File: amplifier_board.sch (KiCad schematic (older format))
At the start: 57 parts, among them J1 VCC (7-14V), J2 AUDIO, J3 GND, J4 speaker, J8 speaker, Q1 SQJ860EP, Q2 Q_NMOS_GSD, Q3 SQJ860EP, U1 AD8038, U2 AD8613, U3 LTC4444-5, U4 AD8468, U5 L7805, U6 LM2776, U7 AD8038, U8 AD8468

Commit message: pcb
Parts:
- removed C1: large, Capacitors_ThroughHole:CP_Radial_D10.0mm_P2.50mm_P5.00mm, symbol amplifier_board-rescue:CP-Device
- removed C3: 100uF, Capacitors_SMD:C_1206_HandSoldering, symbol amplifier_board-rescue:C-Device
- removed J4: speaker, Pin_Headers:Pin_Header_Straight_1x02_Pitch2.54mm, symbol Connector_Generic:Conn_02x01
- removed J8: speaker, Terminal_Blocks:TerminalBlock_bornier-2_P5.08mm, symbol amplifier_board-rescue:Screw_Terminal_01x02-Connector
- removed R1, R2: 220, Resistors_SMD:R_1206_HandSoldering, symbol amplifier_board-rescue:R-Device
- added D4, D5, D6: Schottky, Diodes_SMD:D_SMA-SMB_Universal_Handsoldering, symbol amplifier_board-rescue:D_Schottky-Device
- added J4: A, Wire_Pads:SolderWirePad_single_SMD_5x10mm, symbol Connector:Conn_01x01_Female
- added J5: B, Wire_Pads:SolderWirePad_single_SMD_5x10mm, symbol Connector:Conn_01x01_Female
- added JP1, JP3: Jumper-Device, Pin_Headers:Pin_Header_Straight_1x02_Pitch2.54mm, symbol amplifier_board-rescue:Jumper-Device
- added L2: 10uH, Choke_Toroid_ThroughHole:Choke_Toroid_8x16mm_Vertical, symbol amplifier_board-rescue:L-Device
- added Q4, Q5: SQJ402EP, SMD_Packages:SO-8_PowerPAK_Vishay_Single, symbol amplifier_board-rescue:Si7336ADP-Transistor_FET
- added U9: LTC4444-5, Housings_SSOP:MSOP-8-1EP_3x3mm_Pitch0.65mm, symbol LTC4444-5:LTC4444-5
- C7: value 100uF -> 1.5uF
- C8: value 100uF -> 2.2uF
- J1, J3: footprint Mounting_Holes:MountingHole_4mm_Pad -> Wire_Pads:SolderWirePad_single_SMD_5x10mm
- J2: footprint Pin_Headers:Pin_Header_Straight_1x03_Pitch2.54mm -> Pin_Headers:Pin_Header_Angled_1x02_Pitch2.54mm; symbol amplifier_board-rescue:Conn_01x03-Connector_Generic -> Connector_Generic:Conn_01x02
- Q1, Q3: value SQJ860EP -> SQJ402EP
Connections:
- net GND: now also C7.2, C8.1, D6.2 (A), Q5.1 (S), Q5.2 (S), Q5.3 (S), U9.9 (GND)
- net VCC: now also D4.2 (A), D5.1 (K), Q4.5 (D), U9.3 (VCC)
- net audio_in: now also J2.2 (Pin_2)
- net at Q2.1 (G), U4.1: now also JP1.1; no longer U3.1 (Tinp)
- net at Q2.3 (D), R12.1: now also JP3.1; no longer U3.2 (Binp)
- net at RV3.2, U7.3 (+), U8.4 (-): now also C8.2
- new net: C9.1, J5.1 (Pin_1), L1.2
- new net: JP1.2, U3.1 (Tinp), U9.2 (Binp)
- new net: JP3.2, U3.2 (Binp), U9.1 (Tinp)
- new net: Q5.4 (G), U9.4 (BG)
- new net: C5.1, D5.2 (A), D6.1 (K), L2.1, Q4.1 (S), Q4.2 (S), Q4.3 (S), Q5.5 (D), U9.8 (TS)
- new net: Q4.4 (G), U9.7 (TG)
- new net: C7.1, J4.1 (Pin_1), L2.2
- new net: C5.2, D4.1 (K), U9.6 (VB)
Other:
- moved on the sheet: C16, C25, C6, C9, D1, D2, D3, L1, Q1, Q3, U3

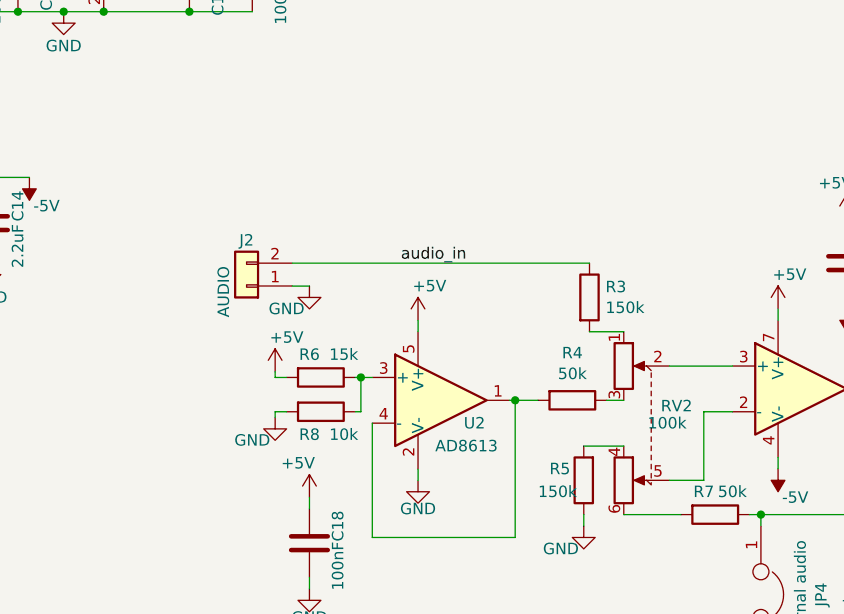
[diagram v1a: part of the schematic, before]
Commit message: pcb improvements
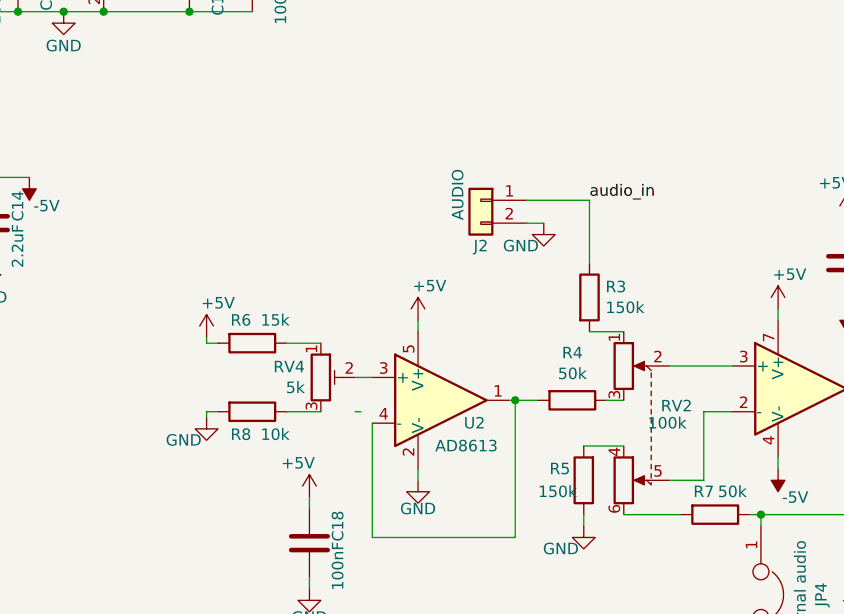
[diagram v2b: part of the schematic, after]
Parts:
- added RV4: 5k, Pin_Headers:Pin_Header_Straight_1x03_Pitch2.54mm, symbol Device:R_POT_TRIM
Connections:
- net GND: now also J2.2 (Pin_2); no longer J2.1 (Pin_1)
- net audio_in: now also J2.1 (Pin_1); no longer J2.2 (Pin_2)
- new net: R6.1, RV4.1
- new net: R8.1, RV4.3
- new net: RV4.2, U2.3 (+)
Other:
- moved on the sheet: J2, R6, R8
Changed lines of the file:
@@
 L amplifier_board-rescue:R-Device R6
 U 1 1 5CA2C628
-P 3375 2825
-F 0 "R6" V 3275 2775 50  0000 C CNN
-F 1 "15k" V 3275 2925 50  0000 C CNN
-F 2 "Resistors_SMD:R_1206_HandSoldering" V 3305 2825 50  0001 C CNN
-F 3 "~" H 3375 2825 50  0001 C CNN
-	1    3375 2825
+P 3075 2675
+F 0 "R6" V 2975 2625 50  0000 C CNN
+F 1 "15k" V 2975 2775 50  0000 C CNN
+F 2 "Resistors_SMD:R_1206_HandSoldering" V 3005 2675 50  0001 C CNN
+F 3 "~" H 3075 2675 50  0001 C CNN
+	1    3075 2675
 	0    1    1    0
 $EndComp
@@
 L amplifier_board-rescue:R-Device R8
 U 1 1 5CA2C63F
-P 3375 2975
-F 0 "R8" V 3475 2925 50  0000 C CNN
-F 1 "10k" V 3475 3075 50  0000 C CNN
-F 2 "Resistors_SMD:R_1206_HandSoldering" V 3305 2975 50  0001 C CNN
-F 3 "~" H 3375 2975 50  0001 C CNN
-	1    3375 2975
+P 3075 2975
+F 0 "R8" V 3175 2925 50  0000 C CNN
+F 1 "10k" V 3175 3075 50  0000 C CNN
+F 2 "Resistors_SMD:R_1206_HandSoldering" V 3005 2975 50  0001 C CNN
+F 3 "~" H 3075 2975 50  0001 C CNN
+	1    3075 2975
 	0    1    1    0
 $EndComp
@@
 L amplifier_board-rescue:GND-power #PWR0121
 U 1 1 5CA2C639
-P 3175 3000
-F 0 "#PWR0121" H 3175 2750 50  0001 C CNN
-F 1 "GND" H 3075 2900 50  0000 C CNN
-F 2 "" H 3175 3000 50  0001 C CNN
-F 3 "" H 3175 3000 50  0001 C CNN
-	1    3175 3000
+P 2875 3000
+F 0 "#PWR0121" H 2875 2750 50  0001 C CNN
+F 1 "GND" H 2775 2900 50  0000 C CNN
+F 2 "" H 2875 3000 50  0001 C CNN
+F 3 "" H 2875 3000 50  0001 C CNN
+	1    2875 3000
 	1    0    0    -1
 $EndComp
@@
 Wire Wire Line
 	4625 2925 4700 2925
-Text Label 3725 2325 0    50   ~ 0
+Text Label 4550 2050 0    50   ~ 0
 audio_in
 $Comp
@@
 L Connector_Generic:Conn_01x02 J2
 U 1 1 5CC7617F
-P 3050 2425
-F 0 "J2" H 3050 2225 50  0000 C CNN
-F 1 "AUDIO" V 3150 2450 50  0000 C CNN
-F 2 "Pin_Headers:Pin_Header_Angled_1x02_Pitch2.54mm" H 3050 2425 50  0001 C CNN
-F 3 "~" H 3050 2425 50  0001 C CNN
-	1    3050 2425
-	-1   0    0    1
+P 4075 2050
+F 0 "J2" H 4075 1850 50  0000 C CNN
+F 1 "AUDIO" V 4175 2075 50  0000 C CNN
+F 2 "Pin_Headers:Pin_Header_Angled_1x02_Pitch2.54mm" H 4075 2050 50  0001 C CNN
+F 3 "~" H 4075 2050 50  0001 C CNN
+	1    4075 2050
+	-1   0    0    -1
 $EndComp
 Wire Wire Line
@@
 L amplifier_board-rescue:+5V-power #PWR0103
 U 1 1 5CAEFEC7
-P 3175 2800
-F 0 "#PWR0103" H 3175 2650 50  0001 C CNN
-F 1 "+5V" H 3225 2950 50  0000 C CNN
-F 2 "" H 3175 2800 50  0001 C CNN
-F 3 "" H 3175 2800 50  0001 C CNN
-	1    3175 2800
-	1    0    0    -1
-$EndComp
-Wire Wire Line
-	3525 2825 3550 2825
-Wire Wire Line
-	3225 2825 3175 2825
-Wire Wire Line
-	3175 2825 3175 2800
-Wire Wire Line
-	3175 2975 3175 3000
-Wire Wire Line
-	3175 2975 3225 2975
+P 2875 2650
+F 0 "#PWR0103" H 2875 2500 50  0001 C CNN
+F 1 "+5V" H 2925 2800 50  0000 C CNN
+F 2 "" H 2875 2650 50  0001 C CNN
+F 3 "" H 2875 2650 50  0001 C CNN
+	1    2875 2650
+	1    0    0    -1
+$EndComp
+Wire Wire Line
+	2925 2675 2875 2675
+Wire Wire Line
+	2875 2675 2875 2650
+Wire Wire Line
+	2875 2975 2875 3000
+Wire Wire Line
+	2875 2975 2925 2975
 Wire Wire Line
 	3525 2975 3550 2975
-Wire Wire Line
-	3550 2975 3550 2825
-Connection ~ 3550 2825
-Wire Wire Line
-	3550 2825 3600 2825
 $Comp
 L amplifier_board-rescue:GND-power #PWR0104
@@
 Connection ~ 7475 4300
 Wire Wire Line
-	3250 2425 3325 2425
-Wire Wire Line
-	3250 2325 4550 2325
+	4275 2150 4350 2150
 $Comp
 L amplifier_board-rescue:GND-power #PWR0102
 U 1 1 5CD7ECEA
-P 3325 2425
-F 0 "#PWR0102" H 3325 2175 50  0001 C CNN
-F 1 "GND" H 3225 2325 50  0000 C CNN
-F 2 "" H 3325 2425 50  0001 C CNN
-F 3 "" H 3325 2425 50  0001 C CNN
-	1    3325 2425
-	1    0    0    -1
-$EndComp
+P 4350 2150
+F 0 "#PWR0102" H 4350 1900 50  0001 C CNN
+F 1 "GND" H 4250 2050 50  0000 C CNN
+F 2 "" H 4350 2150 50  0001 C CNN
+F 3 "" H 4350 2150 50  0001 C CNN
+	1    4350 2150
+	1    0    0    -1
+$EndComp
+$Comp
+L Device:R_POT_TRIM RV4
+U 1 1 5CCE2B00
+P 3375 2825
+F 0 "RV4" H 3305 2871 50  0000 R CNN
+F 1 "5k" H 3305 2780 50  0000 R CNN
+F 2 "Pin_Headers:Pin_Header_Straight_1x03_Pitch2.54mm" H 3375 2825 50  0001 C CNN
+F 3 "~" H 3375 2825 50  0001 C CNN
+	1    3375 2825
+	1    0    0    -1
+$EndComp
+Wire Wire Line
+	3525 2825 3600 2825
+Wire Wire Line
+	3225 2675 3375 2675
+Wire Wire Line
+	3225 2975 3375 2975
+Wire Wire Line
+	4275 2050 4550 2050
+Wire Wire Line
+	4550 2325 4550 2050
 $EndSCHEMATC
